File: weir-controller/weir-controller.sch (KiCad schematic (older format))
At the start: 41 parts, among them J1 Screw_Terminal_01x02, J2 Screw_Terminal_01x04, J3 Screw_Terminal_01x04, J4 USB_B_Mini, J5 Wurth_74980104400, J6 Screw_Terminal_01x02, Q1 PSMN0R7-25YLD, Q2 PSMN0R7-25YLD, Q3 PSMN0R7-25YLD, Q4 PSMN0R7-25YLD, SW1 SW_Push, U1 ESP32-WROOM-32U, U2 DP83825IRMQR, U3 CP2102N-A01-GQFN24, U4 TL1963A-33DCYR

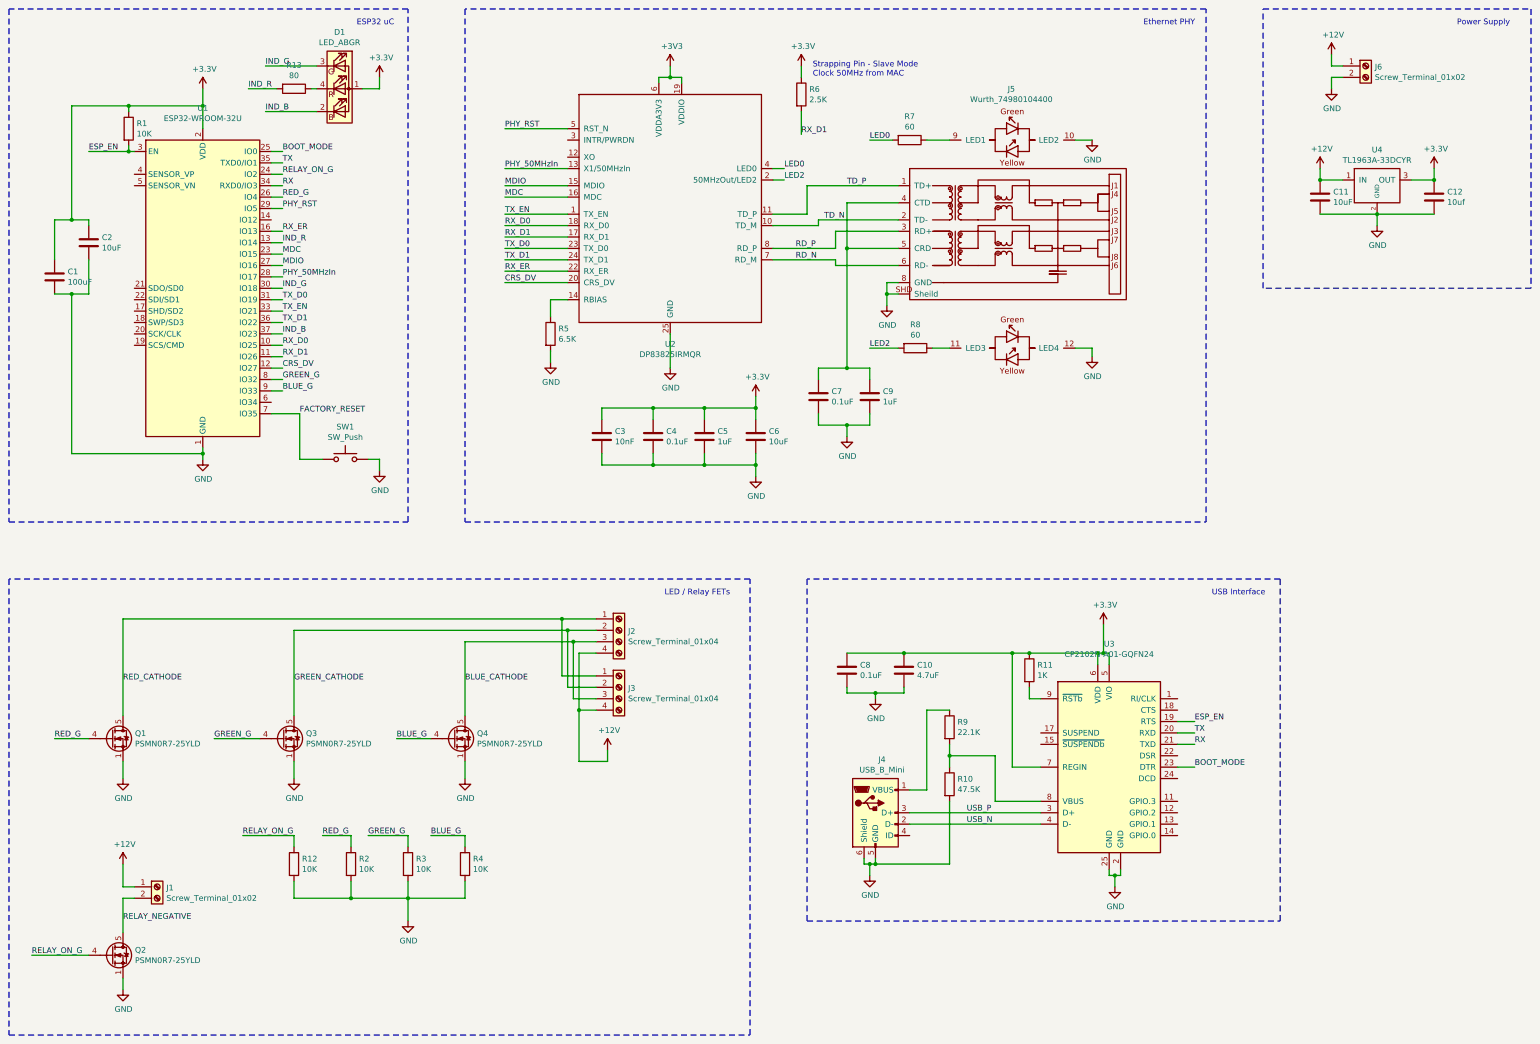
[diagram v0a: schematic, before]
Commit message: v1.1.1
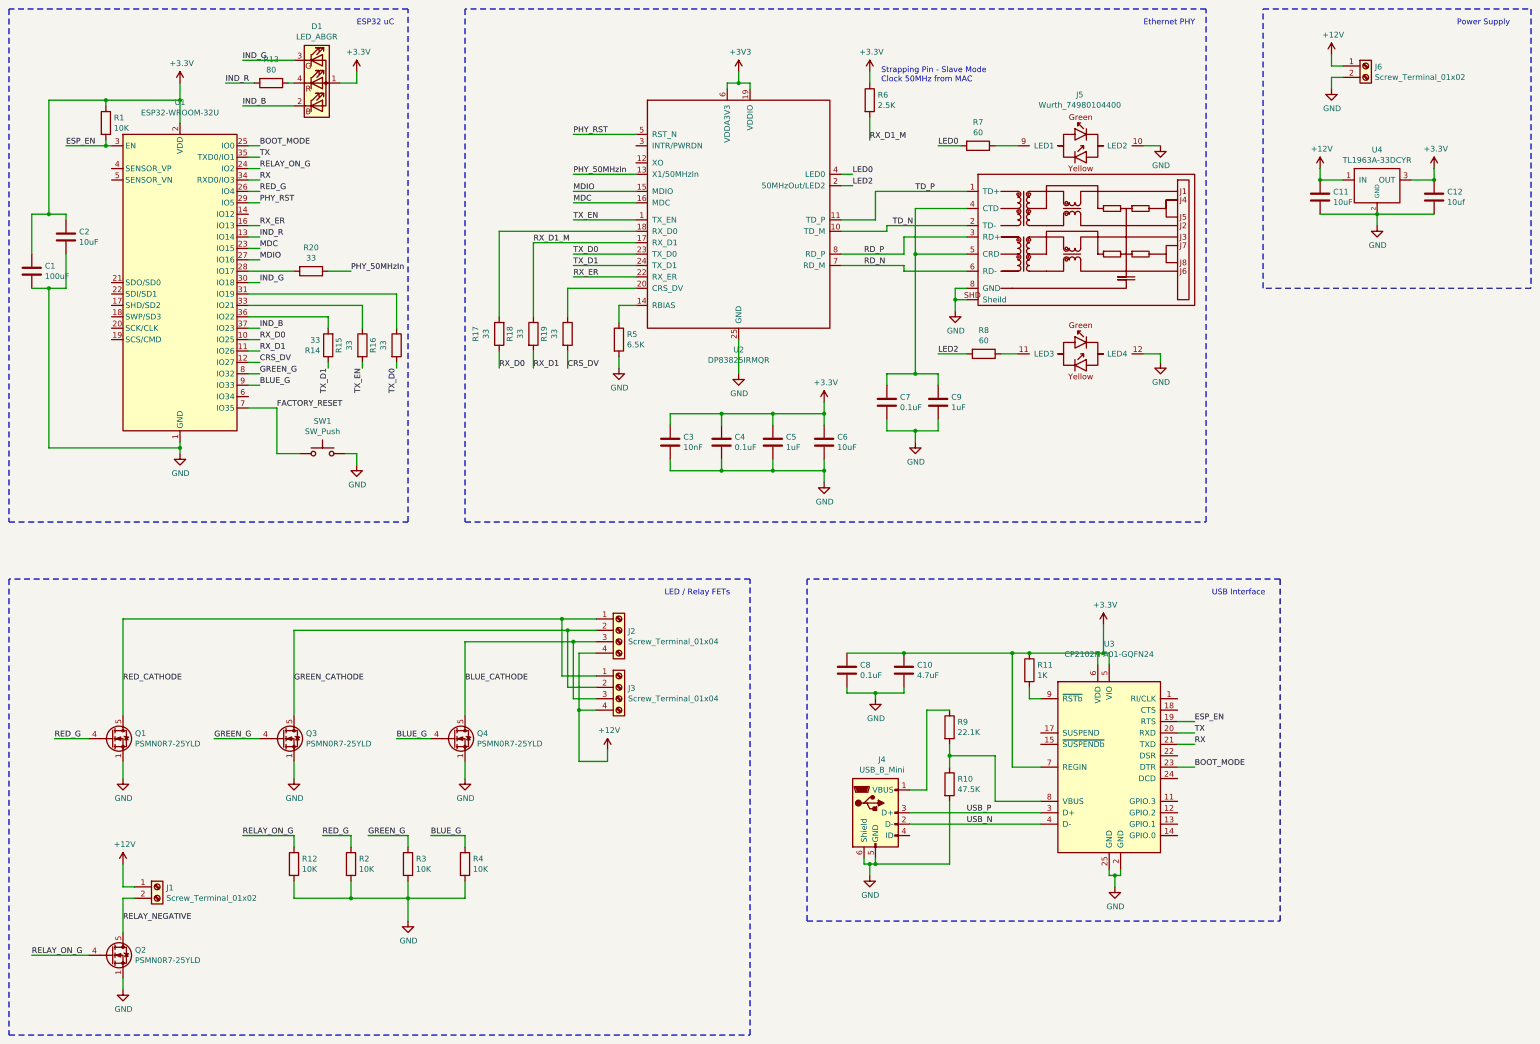
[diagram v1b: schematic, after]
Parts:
- added R14, R15, R16, R17, R18, R19, R20: 33, Resistor_SMD:R_0805_2012Metric_Pad1.15x1.40mm_HandSolder, symbol Device:R
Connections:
- net CRS_DV: now also R19.2; no longer U2.20 (CRS_DV)
- net PHY_50MHzIn: now also R20.1; no longer U1.28 (IO17)
- net RX_D0: now also R17.1; no longer U2.18 (RX_D0)
- net RX_D1: now also R18.2; no longer R6.2, U2.17 (RX_D1)
- net TX_D0: now also R16.2; no longer U1.31 (IO19)
- net TX_D1: now also R14.1; no longer U1.36 (IO22)
- net TX_EN: now also R15.2; no longer U1.33 (IO21)
- new net: R20.2, U1.28 (IO17)
- new net: R16.1, U1.31 (IO19)
- new net: R15.1, U1.33 (IO21)
- new net: R14.2, U1.36 (IO22)
- new net: R17.2, U2.18 (RX_D0)
- new net: R19.1, U2.20 (CRS_DV)
- new net RX_D1_M: R18.1, R6.2, U2.17 (RX_D1)
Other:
- moved on the sheet: C1, C2, C3, C4, C5, C6, C7, C9, D1, J5, R1, R13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
